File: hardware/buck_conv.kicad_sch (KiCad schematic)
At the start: 8 parts, among them J3 Term_2, J4 Term_2, Q1 TIP120

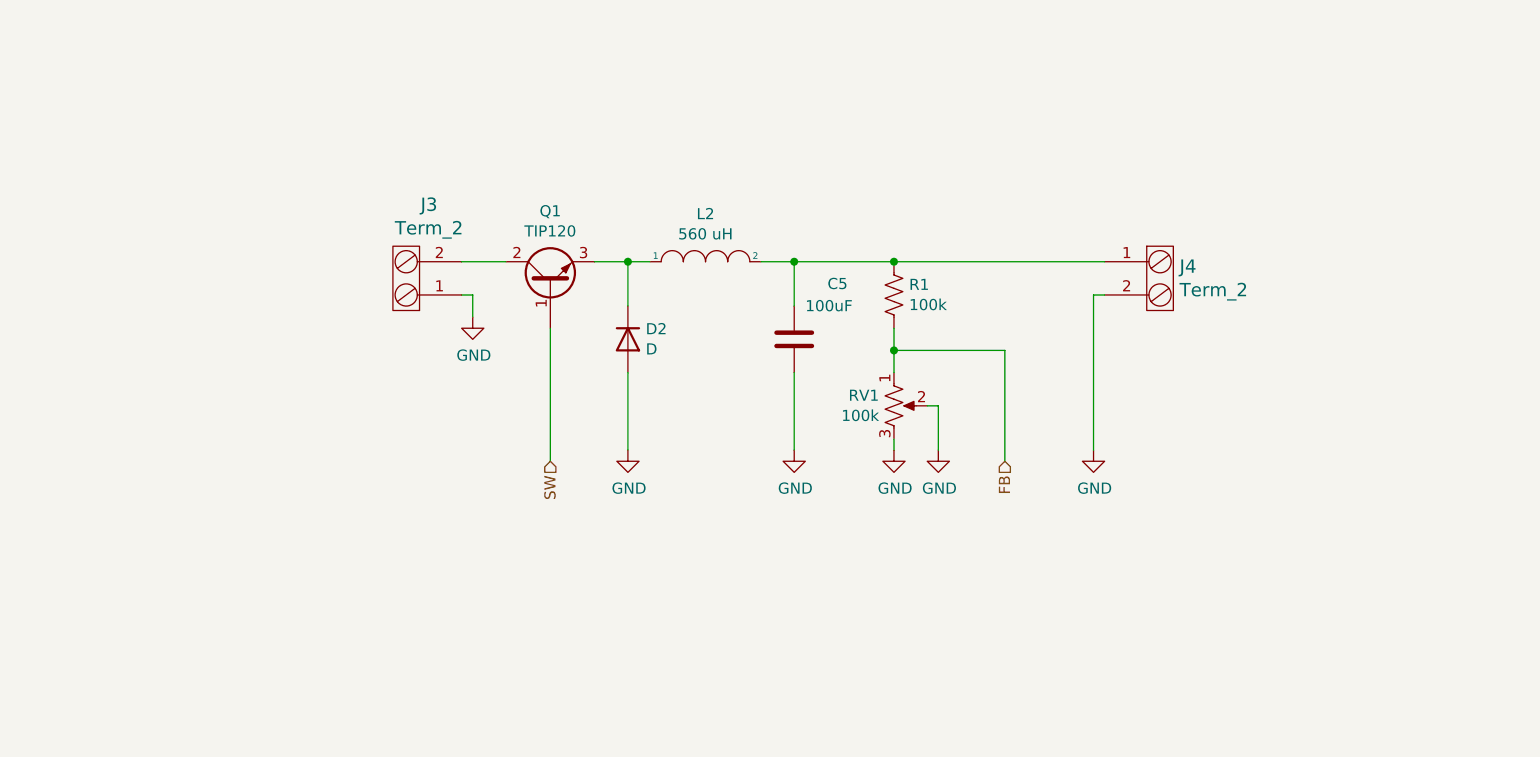
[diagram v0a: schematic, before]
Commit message: JLCPCB order rev-A
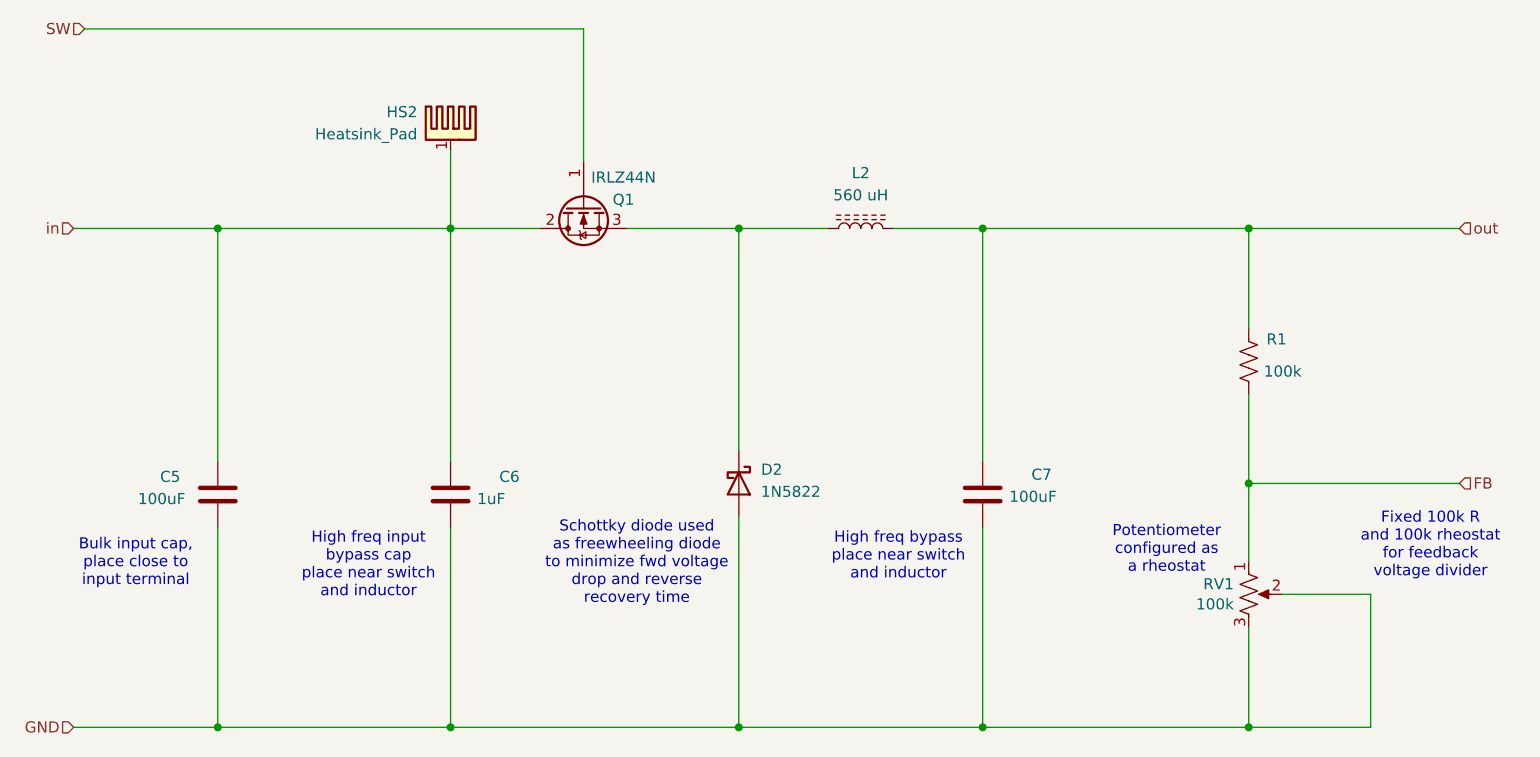
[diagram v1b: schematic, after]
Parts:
- removed D2: D, Diode_THT:D_DO-41_SOD81_P10.16mm_Horizontal, symbol Device:D
- removed J3, J4: Term_2, TerminalBlock_Altech:Altech_AK100_1x02_P5.00mm, symbol BREAD_Slice-rescue:Term_2-OCI_UPL_10_Connectors
- removed L2: 560 uH, Inductor_THT:L_Radial_D28.0mm_P29.20mm, symbol BREAD_Slice-rescue:INDUCTOR-pspice
- removed Q1: TIP120, Package_TO_SOT_THT:TO-220-3_Horizontal_TabUp, symbol BREAD_Slice-rescue:TIP120-OCI_UPL_4_Semiconductors
- added C5: 100uF, Capacitor_THT:C_Radial_D8.0mm_H11.5mm_P3.50mm, symbol Device:C
- added C6: 1uF, Capacitor_SMD:C_1206_3216Metric, symbol Device:C
- added D2: 1N5822, Diode_THT:D_DO-201AD_P15.24mm_Horizontal, symbol Diode:1N5822
- added HS2: Heatsink_Pad, KML-Custom:Thermal Pad, symbol Mechanical:Heatsink_Pad
- added L2: 560 uH, Inductor_THT:L_Radial_D27.9mm_P19.05mm_Vishay_IHB-3, symbol Device:L_Ferrite
- added Q1: IRLZ44N, Package_TO_SOT_THT:TO-220-3_Horizontal_TabDown, symbol Transistor_FET:IRLZ44N
- renumbered C5 to C7
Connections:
- net GND: now also C5.2, C6.2, D2.2 (A)
- net SW: now also Q1.1 (G)
- net out: now reaches C7.1, R1.1
- net out: now also L2.2
- new net: D2.1 (K), L2.1, Q1.3 (S)
- new net in: C5.1, C6.1, HS2.1, Q1.2 (D)
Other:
- note added: "Bulk input cap, place close to input terminal"
- note added: "Fixed 100k R and 100k rheostat for feedback voltage divider"
- note added: "High freq bypass place near switch and inductor"
- note added: "High freq input bypass cap place near switch and inductor"
- note added: "Potentiometer configured as a rheostat"
- note added: "Schottky diode used as freewheeling diode to minimize fwd voltage drop and reverse recovery time"
- moved on the sheet: C7, R1, RV1
